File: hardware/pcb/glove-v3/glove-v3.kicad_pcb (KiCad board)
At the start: 4 copper layers, 79 x 35 mm, 43 parts, among them U1 XIAO-ESP32C3, U2 CD74HC4067M96, U3 2.5x3mm-BUTTON

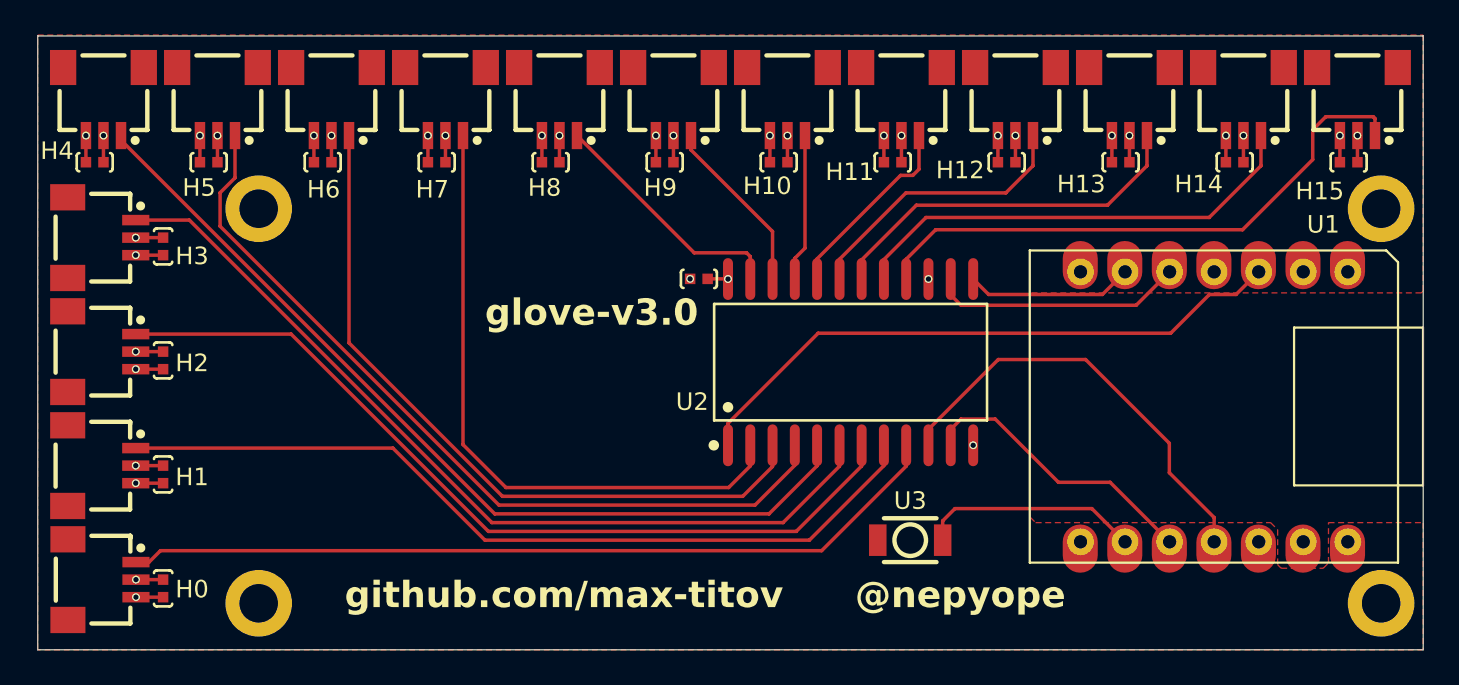
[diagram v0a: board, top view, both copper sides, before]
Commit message: updating v3.1
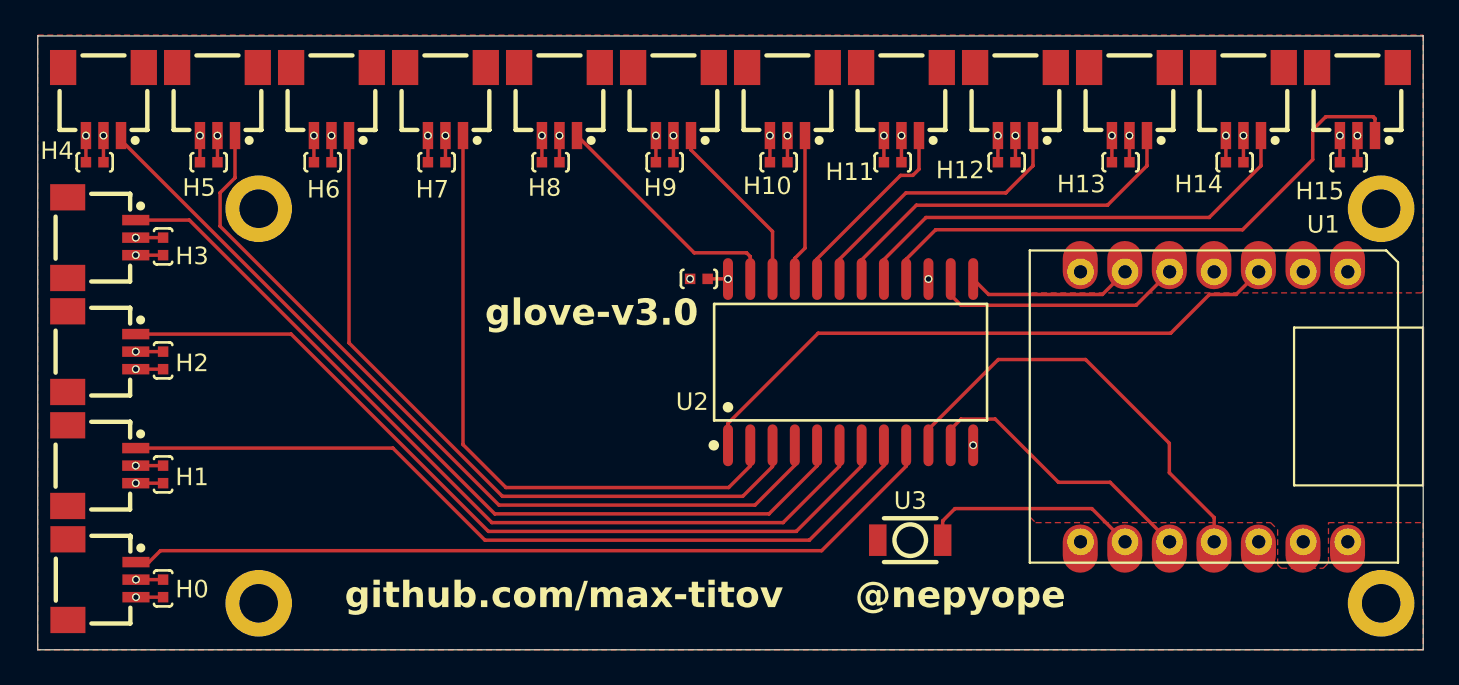
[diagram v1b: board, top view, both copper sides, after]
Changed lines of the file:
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@@
 		(fp_arc
 			(start 1.025 0.368934)
-			(mid 0.981065 0.475001)
+			(mid 0.981065 0.474997)
 			(end 0.875 0.518934)
 			(stroke
@@
 		(fp_arc
 			(start 0.875 -0.518934)
-			(mid 0.98107 -0.475006)
+			(mid 0.981073 -0.475006)
 			(end 1.025 -0.368934)
 			(stroke
@@
 		(fp_arc
 			(start 1.025 0.368934)
-			(mid 0.981065 0.475001)
+			(mid 0.981065 0.474997)
 			(end 0.875 0.518934)
 			(stroke
@@
 		(fp_arc
 			(start 0.875 -0.518934)
-			(mid 0.98107 -0.475006)
+			(mid 0.981073 -0.475006)
 			(end 1.025 -0.368934)
 			(stroke
@@
 		(fp_arc
 			(start 1.025 0.368934)
-			(mid 0.981065 0.475001)
+			(mid 0.981065 0.474997)
 			(end 0.875 0.518934)
 			(stroke
@@
 		(fp_arc
 			(start 0.875 -0.518934)
-			(mid 0.98107 -0.475006)
+			(mid 0.981073 -0.475006)
 			(end 1.025 -0.368934)
 			(stroke
@@
 		(fp_arc
 			(start 1.025 0.368934)
-			(mid 0.981065 0.475001)
+			(mid 0.981065 0.474997)
 			(end 0.875 0.518934)
 			(stroke
@@
 		(fp_arc
 			(start 0.875 -0.518934)
-			(mid 0.98107 -0.475006)
+			(mid 0.981073 -0.475006)
 			(end 1.025 -0.368934)
 			(stroke
@@
 		(fp_arc
 			(start 1.025 0.368934)
-			(mid 0.981065 0.475001)
+			(mid 0.981065 0.474997)
 			(end 0.875 0.518934)
 			(stroke
@@
 		(fp_arc
 			(start 0.875 -0.518934)
-			(mid 0.98107 -0.475006)
+			(mid 0.981073 -0.475006)
 			(end 1.025 -0.368934)
 			(stroke
@@
 		(fp_arc
 			(start 1.025 0.368934)
-			(mid 0.981065 0.475001)
+			(mid 0.981065 0.474997)
 			(end 0.875 0.518934)
 			(stroke
@@
 		(fp_arc
 			(start 0.875 -0.518934)
-			(mid 0.98107 -0.475006)
+			(mid 0.981073 -0.475006)
 			(end 1.025 -0.368934)
 			(stroke
@@
 		(fp_arc
 			(start 1.025 0.368934)
-			(mid 0.981065 0.475001)
+			(mid 0.981065 0.474997)
 			(end 0.875 0.518934)
 			(stroke
@@
 		(fp_arc
 			(start 0.875 -0.518934)
-			(mid 0.98107 -0.475006)
+			(mid 0.981073 -0.475006)
 			(end 1.025 -0.368934)
 			(stroke
@@
 		(fp_arc
 			(start 1.025 0.368934)
-			(mid 0.981065 0.475001)
+			(mid 0.981065 0.474997)
 			(end 0.875 0.518934)
 			(stroke
@@
 		(fp_arc
 			(start 0.875 -0.518934)
-			(mid 0.98107 -0.475006)
+			(mid 0.981073 -0.475006)
 			(end 1.025 -0.368934)
 			(stroke
@@
 		(fp_arc
 			(start 1.025 0.368934)
-			(mid 0.981065 0.475001)
+			(mid 0.981065 0.474997)
 			(end 0.875 0.518934)
 			(stroke
@@
 		(fp_arc
 			(start 0.875 -0.518934)
-			(mid 0.98107 -0.475006)
+			(mid 0.981073 -0.475006)
 			(end 1.025 -0.368934)
 			(stroke
@@
 		(fp_arc
 			(start 1.025 0.368934)
-			(mid 0.981065 0.475001)
+			(mid 0.981065 0.474997)
 			(end 0.875 0.518934)
 			(stroke
@@
 		(fp_arc
 			(start 0.875 -0.518934)
-			(mid 0.98107 -0.475006)
+			(mid 0.981073 -0.475006)
 			(end 1.025 -0.368934)
 			(stroke
@@
 		(fp_arc
 			(start 1.025 0.368934)
-			(mid 0.981065 0.475001)
+			(mid 0.981065 0.474997)
 			(end 0.875 0.518934)
 			(stroke
@@
 		(fp_arc
 			(start 0.875 -0.518934)
-			(mid 0.98107 -0.475006)
+			(mid 0.981073 -0.475006)
 			(end 1.025 -0.368934)
 			(stroke
@@
 		(fp_arc
 			(start 1.025 0.368934)
-			(mid 0.981065 0.475001)
+			(mid 0.981065 0.474997)
 			(end 0.875 0.518934)
 			(stroke
@@
 		(fp_arc
 			(start 0.875 -0.518934)
-			(mid 0.98107 -0.475006)
+			(mid 0.981073 -0.475006)
 			(end 1.025 -0.368934)
 			(stroke
@@
 		(fp_arc
 			(start 1.025 0.368934)
-			(mid 0.981065 0.475001)
+			(mid 0.981065 0.474997)
 			(end 0.875 0.518934)
 			(stroke
@@
 		(fp_arc
 			(start 0.875 -0.518934)
-			(mid 0.98107 -0.475006)
+			(mid 0.981073 -0.475006)
 			(end 1.025 -0.368934)
 			(stroke
@@
 		(fp_arc
 			(start 1.025 0.368934)
-			(mid 0.981065 0.475001)
+			(mid 0.981065 0.474997)
 			(end 0.875 0.518934)
 			(stroke
@@
 		(fp_arc
 			(start 0.875 -0.518934)
-			(mid 0.98107 -0.475006)
+			(mid 0.981073 -0.475006)
 			(end 1.025 -0.368934)
 			(stroke
@@
 		(fp_arc
 			(start 1.025 0.368934)
-			(mid 0.981065 0.475001)
+			(mid 0.981065 0.474997)
 			(end 0.875 0.518934)
 			(stroke
@@
 		(fp_arc
 			(start 0.875 -0.518934)
-			(mid 0.98107 -0.475006)
+			(mid 0.981073 -0.475006)
 			(end 1.025 -0.368934)
 			(stroke
@@
 		(fp_arc
 			(start 1.025 0.368934)
-			(mid 0.981065 0.475001)
+			(mid 0.981065 0.474997)
 			(end 0.875 0.518934)
 			(stroke
@@
 		(fp_arc
 			(start 0.875 -0.518934)
-			(mid 0.98107 -0.475006)
+			(mid 0.981073 -0.475006)
 			(end 1.025 -0.368934)
 			(stroke
@@
 		(fp_arc
 			(start 1.025 0.368934)
-			(mid 0.981065 0.475001)
+			(mid 0.981065 0.474997)
 			(end 0.875 0.518934)
 			(stroke
@@
 		(fp_arc
 			(start 0.875 -0.518934)
-			(mid 0.98107 -0.475006)
+			(mid 0.981073 -0.475006)
 			(end 1.025 -0.368934)
 			(stroke
